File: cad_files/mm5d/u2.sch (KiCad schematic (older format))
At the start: 1 part

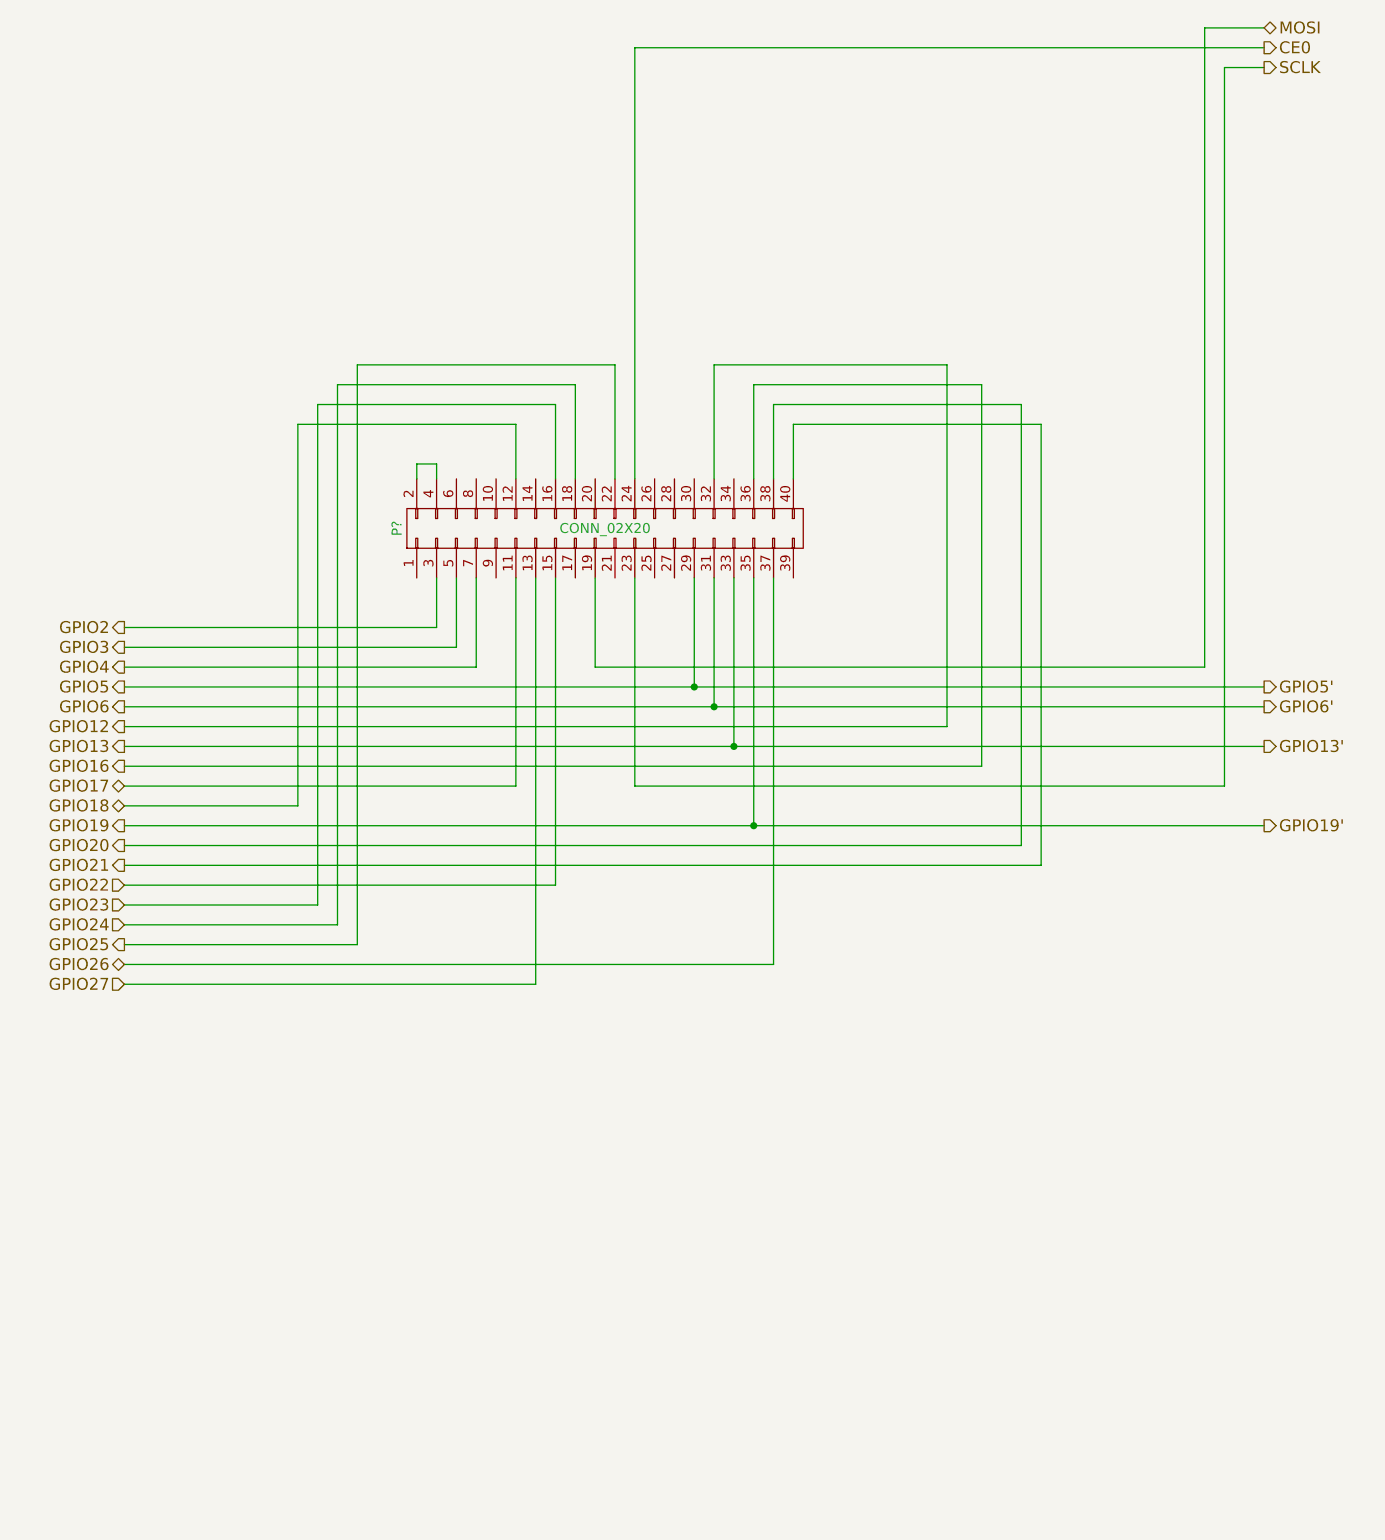
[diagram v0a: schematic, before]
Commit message: 190922
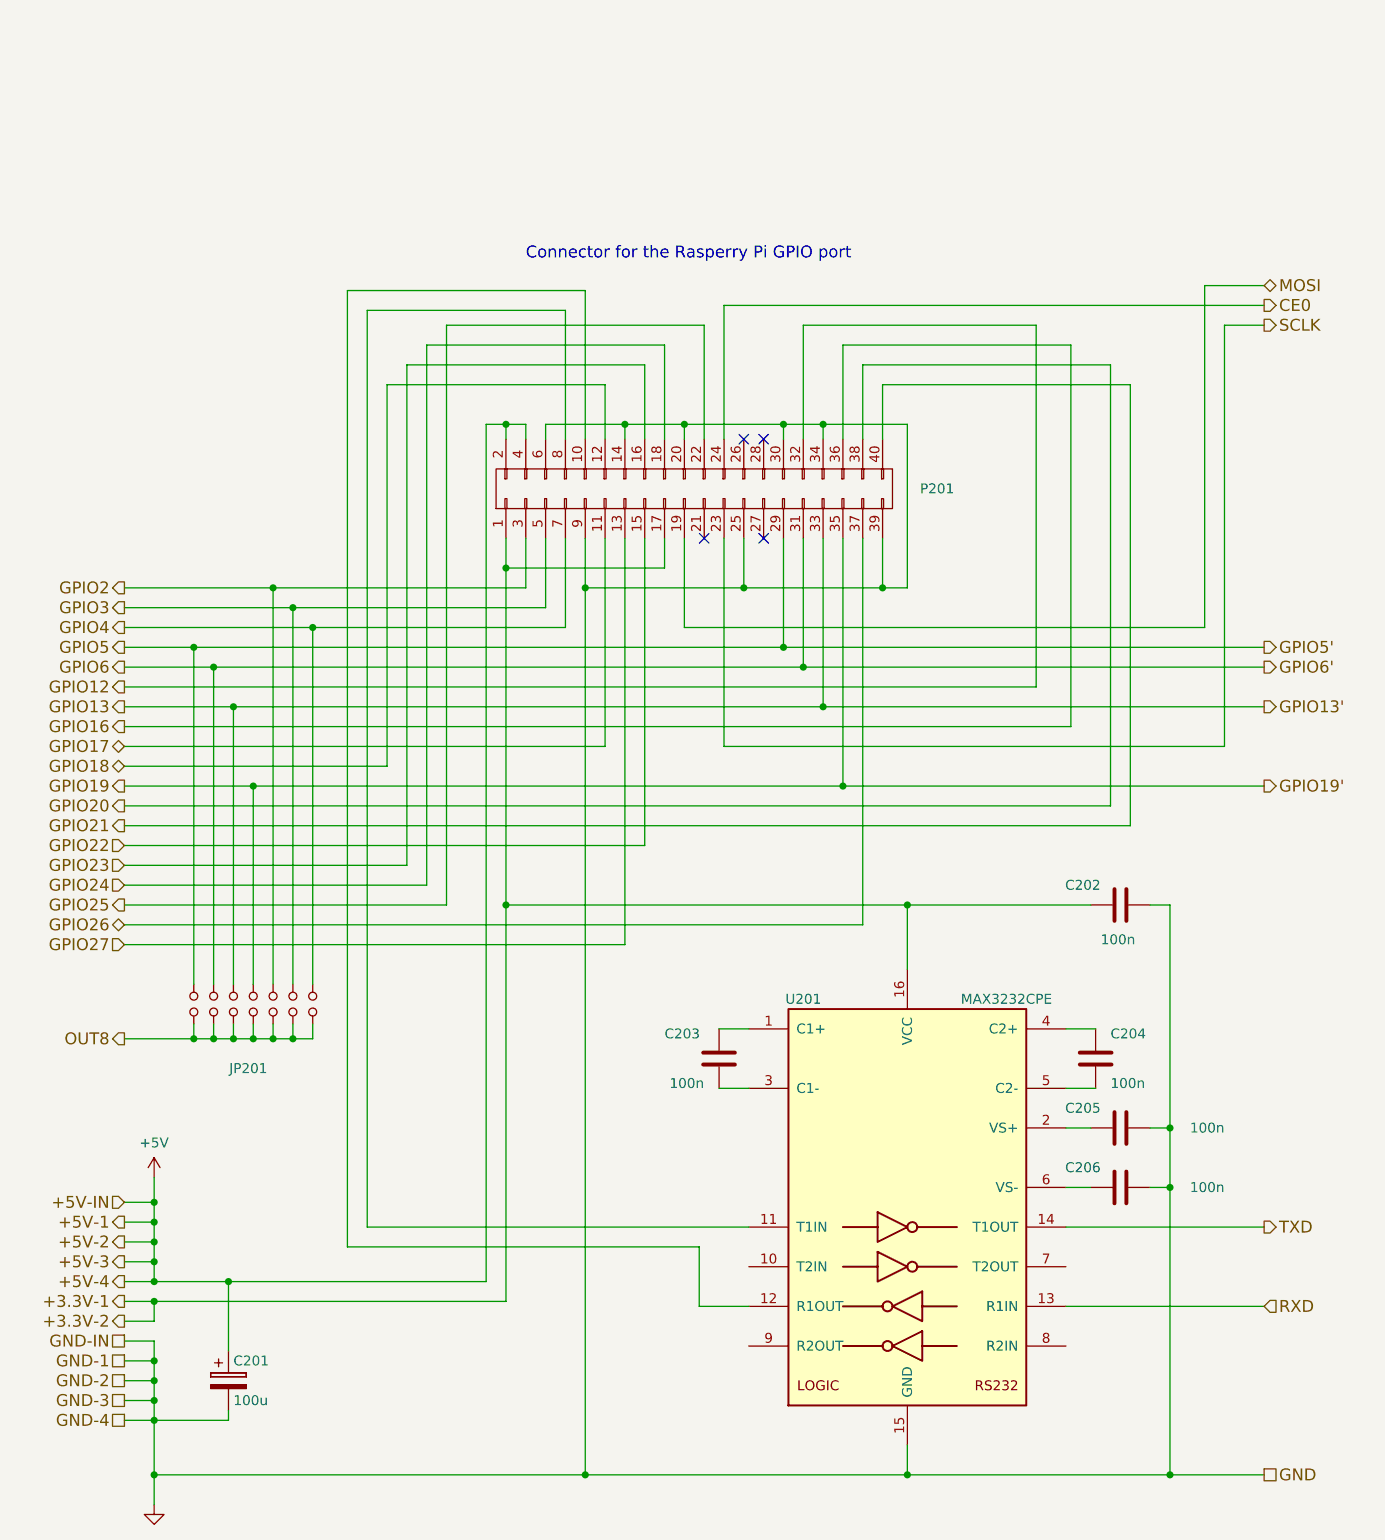
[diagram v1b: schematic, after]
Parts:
- added C201: 100u, symbol CP
- added C202, C203, C204, C205, C206: 100n, symbol C
- added JP201, JP? (x6): Jumper_NO_Small, symbol Jumper_NO_Small
- added U201: MAX3232CPE, symbol MAX232
- gave numbers to parts that had none: 1
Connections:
- net GPIO13: now also JP?.1
- net GPIO19: now also JP?.1
- net GPIO2: now also JP?.1
- net GPIO3: now also JP?.1
- net GPIO4: now also JP?.1
- net GPIO5: now also JP201.1
- net GPIO6: now also JP?.1
- net +3.3V-1: now reaches P201.1 (P1)
- net +3.3V-1: now also P201.17 (P17), C202.1, U201.16 (VCC)
- net at P201.10 (P10): now also U201.12 (R1OUT)
- net GND: now reaches P201.14 (P14)
- net GND: now also P201.20 (P20), P201.25 (P25), P201.30 (P30), P201.34 (P34), P201.39 (P39), P201.6 (P6), P201.9 (P9), C201.2, C202.2, C205.2, C206.2, U201.15 (GND)
- net +5V: now reaches P201.2 (P2), P201.4 (P4)
- net +5V: now also C201.1
- net at P201.8 (P8): now also U201.11 (T1IN)
- new net: C203.1, U201.1 (C1+)
- new net: C205.1, U201.2 (VS+)
- new net: C203.2, U201.3 (C1-)
- new net: C204.1, U201.4 (C2+)
- new net: C204.2, U201.5 (C2-)
- new net: C206.1, U201.6 (VS-)
- new net OUT8: JP201.2, JP?.2, JP?.2, JP?.2, JP?.2, JP?.2, JP?.2
- new net RXD: U201.13 (R1IN)
- new net TXD: U201.14 (T1OUT)
- no-connect marks 0 -> 4
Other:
- note added: "Connector for the Rasperry Pi GPIO port"
- moved on the sheet: P201
